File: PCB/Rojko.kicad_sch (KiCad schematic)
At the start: 30 parts, among them IC1 STM32L051C8T6, IC2 BQ25186DLHR, IC3 AP63203WU-7, J1 Conn_01x10_Socket, J2 Conn_01x10_Socket, SW1 SW_MEC_5G, Y1 32,768k

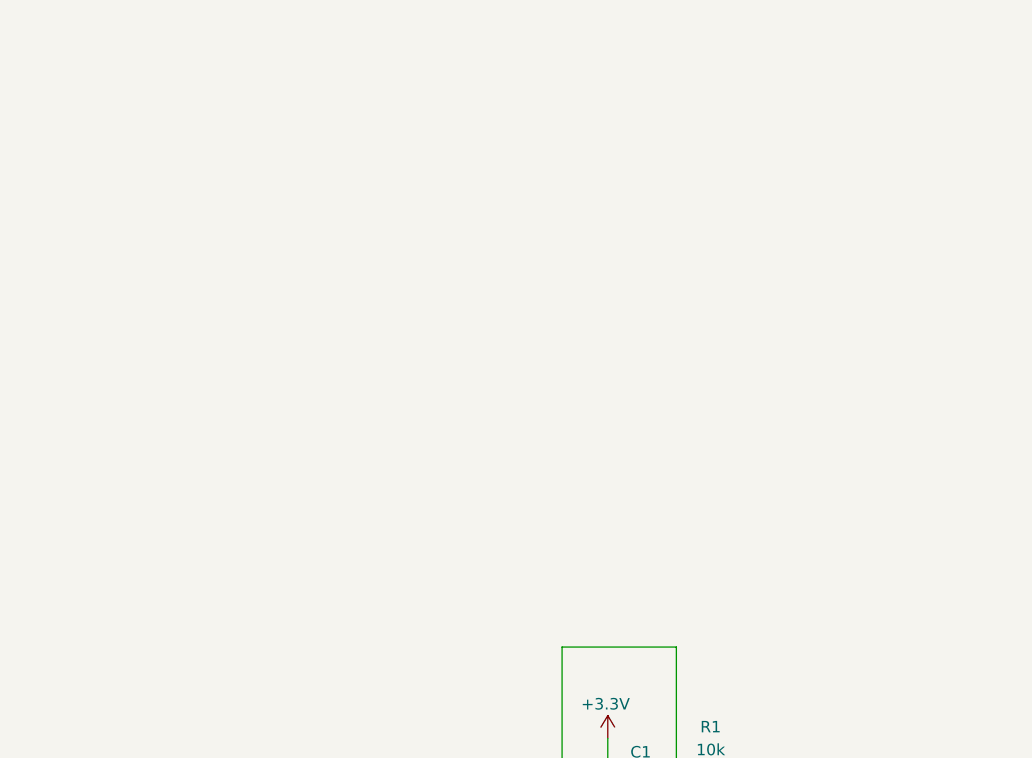
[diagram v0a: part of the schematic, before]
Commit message: ble add
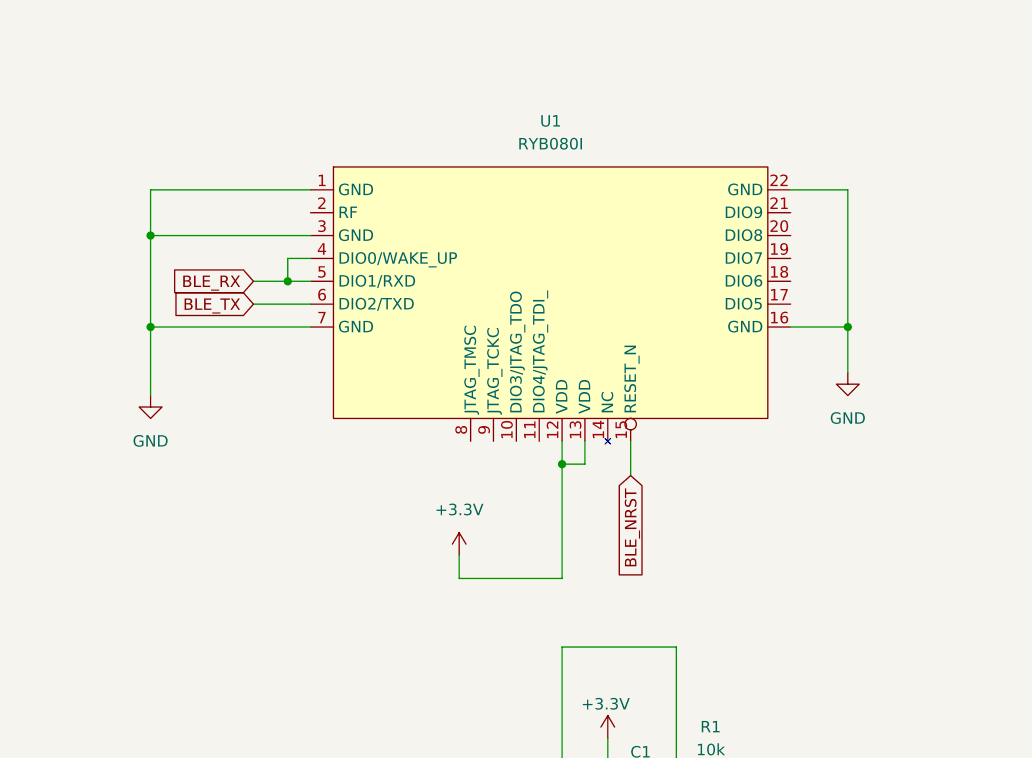
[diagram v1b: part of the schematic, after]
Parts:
- added U1: RYB080I, symbol RYB080l:RYB080i
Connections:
- net +3.3V: now also U1.12 (VDD), U1.13 (VDD)
- net GND: now also U1.1 (GND), U1.16 (GND), U1.22 (GND), U1.3 (GND), U1.7 (GND)
- new net BLE_NRST: U1.15 (RESET_N)
- new net BLE_RX: U1.4 (DIO0/WAKE_UP), U1.5 (DIO1/RXD)
- new net BLE_TX: U1.6 (DIO2/TXD)
